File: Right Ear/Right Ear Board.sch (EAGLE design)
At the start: 6 parts, among them J1 502585-0470

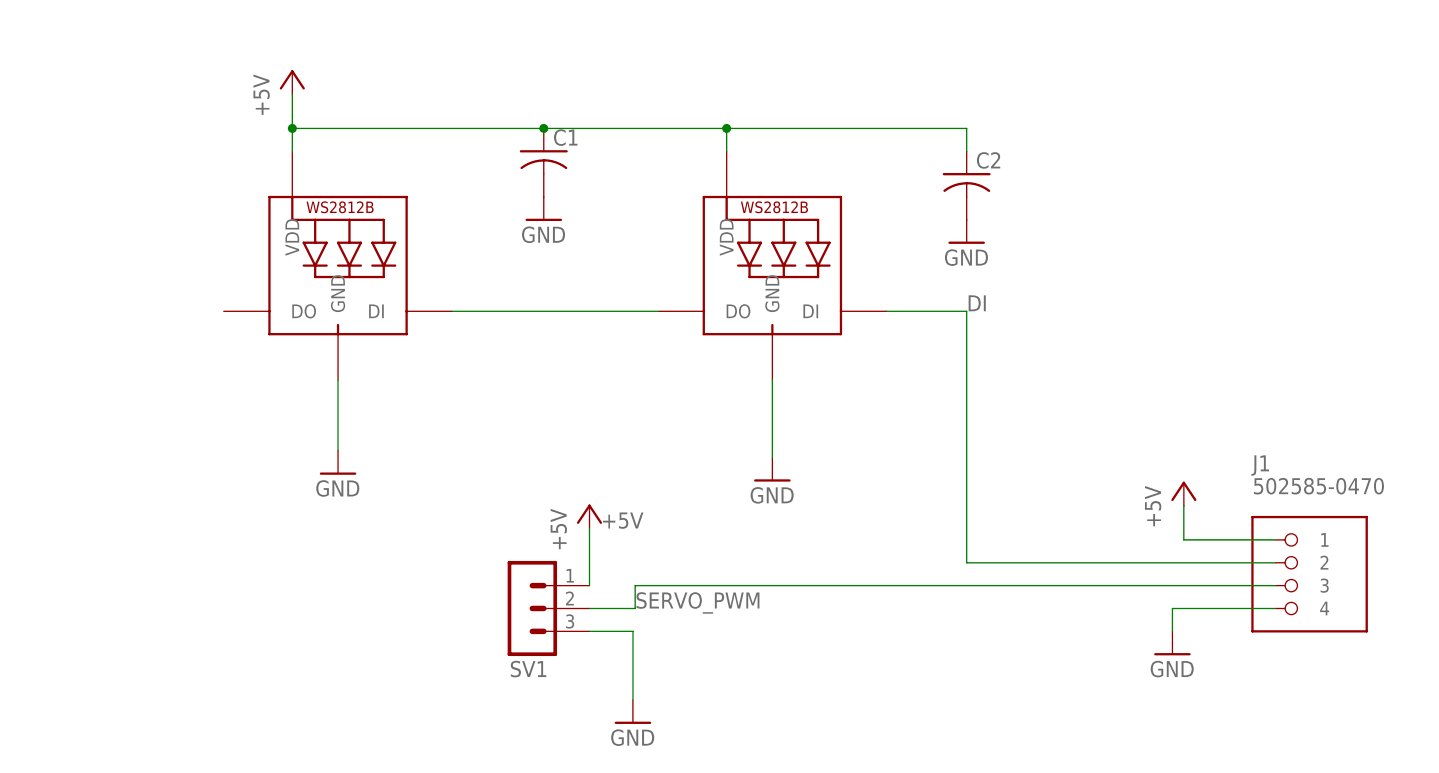
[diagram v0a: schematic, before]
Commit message: Update right ear boards
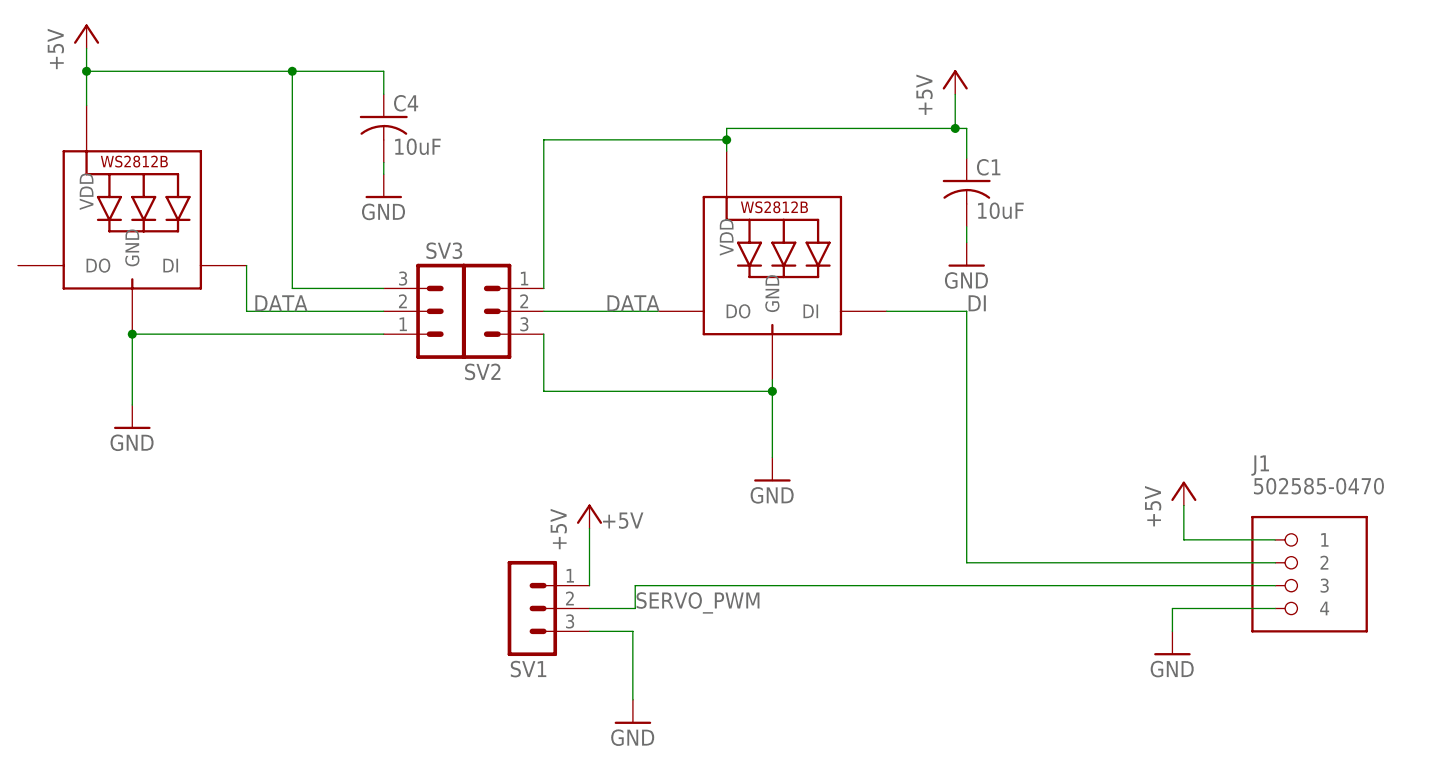
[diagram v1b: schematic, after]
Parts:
- removed C2: (no value), rcl:C-USC0402
- added C4: 10uF, rcl:C-USC0603K
- added SV2, SV3: (no value), con-lstb:MA03-1
- C1: value (none) -> 10uF; device rcl:C-USC0402 -> rcl:C-USC0603K; PARTNO (none) -> GRM188R61A106KE69D
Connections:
- removed net N$1: LED1.DO, LED7.DI
- new net DATA: LED1.DO, LED7.DI, SV2.2, SV3.2
- net +5V: now also C4.1, SV2.1, SV3.3; no longer C2.1
- net GND: now also C4.2, SV2.3, SV3.1; no longer C2.2
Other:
- moved on the sheet: C1
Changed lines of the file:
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@@
 <?xml version="1.0" encoding="utf-8"?>
 <!DOCTYPE eagle SYSTEM "eagle.dtd">
-<eagle version="8.6.0">
+<eagle version="8.5.0">
 <drawing>
 <settings>
@@
 <part name="LED7" library="adafruit" deviceset="WS2812B" device="5050"/>
 <part name="LED1" library="adafruit" deviceset="WS2812B" device="5050"/>
-<part name="C1" library="rcl" library_urn="urn:adsk.eagle:library:334" deviceset="C-US" device="C0402" package3d_urn="urn:adsk.eagle:package:23626/1"/>
 <part name="GND20" library="supply1" deviceset="GND" device=""/>
-<part name="C2" library="rcl" library_urn="urn:adsk.eagle:library:334" deviceset="C-US" device="C0402" package3d_urn="urn:adsk.eagle:package:23626/1"/>
 <part name="GND1" library="supply1" deviceset="GND" device=""/>
 <part name="J1" library="FormE" deviceset="MOLEX_CLICKMATE-4-R/A" device="" value="502585-0470"/>
@@
 <part name="P+2" library="supply1" library_urn="urn:adsk.eagle:library:371" deviceset="+5V" device=""/>
 <part name="P+3" library="supply1" library_urn="urn:adsk.eagle:library:371" deviceset="+5V" device=""/>
+<part name="SV2" library="con-lstb" library_urn="urn:adsk.eagle:library:162" deviceset="MA03-1" device="" package3d_urn="urn:adsk.eagle:package:8339/1"/>
+<part name="SV3" library="con-lstb" library_urn="urn:adsk.eagle:library:162" deviceset="MA03-1" device="" package3d_urn="urn:adsk.eagle:package:8339/1"/>
+<part name="C4" library="rcl" deviceset="C-US" device="C0603K" value="10uF">
+<attribute name="PARTNO" value="GRM188R61A106KE69D"/>
+</part>
+<part name="C1" library="rcl" deviceset="C-US" device="C0603K" value="10uF">
+<attribute name="PARTNO" value="GRM188R61A106KE69D"/>
+</part>
+<part name="P+4" library="supply1" library_urn="urn:adsk.eagle:library:371" deviceset="+5V" device=""/>
 </parts>
 <sheets>
@@
 <instances>
 <instance part="SV1" gate="G$1" x="78.74" y="46.99" rot="MR180"/>
-<instance part="LED7" gate="G$1" x="58.42" y="82.55" rot="MR0"/>
+<instance part="LED7" gate="G$1" x="35.56" y="87.63" rot="MR0"/>
 <instance part="LED1" gate="G$1" x="106.68" y="82.55" rot="MR0"/>
-<instance part="C1" gate="G$1" x="81.28" y="97.79"/>
-<instance part="GND20" gate="1" x="81.28" y="90.17"/>
-<instance part="C2" gate="G$1" x="128.27" y="95.25"/>
-<instance part="GND1" gate="1" x="128.27" y="87.63"/>
+<instance part="GND20" gate="1" x="63.5" y="92.71"/>
+<instance part="GND1" gate="1" x="128.27" y="85.09"/>
 <instance part="J1" gate="G$1" x="165.1" y="49.53"/>
-<instance part="GND2" gate="1" x="58.42" y="61.976"/>
+<instance part="GND2" gate="1" x="35.56" y="67.056"/>
 <instance part="GND3" gate="1" x="106.68" y="61.214"/>
 <instance part="GND4" gate="1" x="91.186" y="34.29"/>
 <instance part="GND5" gate="1" x="151.13" y="41.91"/>
 <instance part="P+1" gate="1" x="152.4" y="60.96"/>
-<instance part="P+2" gate="1" x="53.34" y="106.68"/>
+<instance part="P+2" gate="1" x="30.48" y="111.76"/>
 <instance part="P+3" gate="1" x="86.36" y="58.42"/>
+<instance part="SV2" gate="G$1" x="73.66" y="80.01" rot="MR180"/>
+<instance part="SV3" gate="G$1" x="71.12" y="80.01" rot="MR0"/>
+<instance part="C4" gate="G$1" x="63.5" y="101.6">
+<attribute name="PARTNO" x="63.5" y="101.6" size="1.778" layer="96" display="off"/>
+</instance>
+<instance part="C1" gate="G$1" x="128.27" y="94.488">
+<attribute name="PARTNO" x="128.27" y="94.488" size="1.778" layer="96" display="off"/>
+</instance>
+<instance part="P+4" gate="1" x="127" y="106.68"/>
 </instances>
 <busses>
@@
 </segment>
 <segment>
-<pinref part="C1" gate="G$1" pin="1"/>
-<pinref part="LED7" gate="G$1" pin="VDD"/>
-<wire x1="53.34" y1="97.79" x2="53.34" y2="100.33" width="0.1524" layer="91"/>
-<wire x1="53.34" y1="100.33" x2="53.34" y2="104.14" width="0.1524" layer="91"/>
-<wire x1="81.28" y1="100.33" x2="53.34" y2="100.33" width="0.1524" layer="91"/>
-<junction x="53.34" y="100.33"/>
-<pinref part="LED1" gate="G$1" pin="VDD"/>
-<wire x1="101.6" y1="97.79" x2="101.6" y2="100.33" width="0.1524" layer="91"/>
-<wire x1="81.28" y1="100.33" x2="101.6" y2="100.33" width="0.1524" layer="91"/>
-<junction x="81.28" y="100.33"/>
-<junction x="101.6" y="100.33"/>
-<pinref part="C2" gate="G$1" pin="1"/>
-<wire x1="101.6" y1="100.33" x2="128.27" y2="100.33" width="0.1524" layer="91"/>
-<wire x1="128.27" y1="100.33" x2="128.27" y2="97.79" width="0.1524" layer="91"/>
-<pinref part="P+2" gate="1" pin="+5V"/>
-</segment>
-<segment>
 <pinref part="J1" gate="G$1" pin="1"/>
 <wire x1="162.56" y1="54.61" x2="152.4" y2="54.61" width="0.1524" layer="91"/>
@@
 <pinref part="P+1" gate="1" pin="+5V"/>
 </segment>
+<segment>
+<wire x1="128.27" y1="100.33" x2="128.27" y2="97.028" width="0.1524" layer="91"/>
+<wire x1="101.6" y1="100.33" x2="127" y2="100.33" width="0.1524" layer="91"/>
+<pinref part="LED1" gate="G$1" pin="VDD"/>
+<wire x1="127" y1="100.33" x2="128.27" y2="100.33" width="0.1524" layer="91"/>
+<wire x1="101.6" y1="97.79" x2="101.6" y2="99.06" width="0.1524" layer="91"/>
+<pinref part="SV2" gate="G$1" pin="1"/>
+<wire x1="101.6" y1="99.06" x2="101.6" y2="100.33" width="0.1524" layer="91"/>
+<wire x1="81.28" y1="82.55" x2="81.28" y2="99.06" width="0.1524" layer="91"/>
+<wire x1="81.28" y1="99.06" x2="101.6" y2="99.06" width="0.1524" layer="91"/>
+<junction x="101.6" y="99.06"/>
+<pinref part="C1" gate="G$1" pin="1"/>
+<pinref part="P+4" gate="1" pin="+5V"/>
+<wire x1="127" y1="104.14" x2="127" y2="100.33" width="0.1524" layer="91"/>
+<junction x="127" y="100.33"/>
+</segment>
+<segment>
+<pinref part="LED7" gate="G$1" pin="VDD"/>
+<pinref part="P+2" gate="1" pin="+5V"/>
+<wire x1="30.48" y1="102.87" x2="30.48" y2="106.68" width="0.1524" layer="91"/>
+<pinref part="C4" gate="G$1" pin="1"/>
+<wire x1="30.48" y1="106.68" x2="30.48" y2="109.22" width="0.1524" layer="91"/>
+<wire x1="63.5" y1="104.14" x2="63.5" y2="106.68" width="0.1524" layer="91"/>
+<wire x1="63.5" y1="106.68" x2="53.34" y2="106.68" width="0.1524" layer="91"/>
+<junction x="30.48" y="106.68"/>
+<pinref part="SV3" gate="G$1" pin="3"/>
+<wire x1="53.34" y1="106.68" x2="30.48" y2="106.68" width="0.1524" layer="91"/>
+<wire x1="63.5" y1="82.55" x2="53.34" y2="82.55" width="0.1524" layer="91"/>
+<wire x1="53.34" y1="82.55" x2="53.34" y2="106.68" width="0.1524" layer="91"/>
+<junction x="53.34" y="106.68"/>
+</segment>
 </net>
 <net name="GND" class="0">
-<segment>
-<pinref part="C1" gate="G$1" pin="2"/>
-<pinref part="GND20" gate="1" pin="GND"/>
-</segment>
-<segment>
-<pinref part="C2" gate="G$1" pin="2"/>
-<pinref part="GND1" gate="1" pin="GND"/>
-</segment>
 <segment>
 <pinref part="J1" gate="G$1" pin="4"/>
@@
 <pinref part="LED7" gate="G$1" pin="GND"/>
 <pinref part="GND2" gate="1" pin="GND"/>
-<wire x1="58.42" y1="72.39" x2="58.42" y2="64.516" width="0.1524" layer="91"/>
+<wire x1="35.56" y1="77.47" x2="35.56" y2="69.596" width="0.1524" layer="91"/>
+<pinref part="SV3" gate="G$1" pin="1"/>
+<wire x1="63.5" y1="77.47" x2="35.56" y2="77.47" width="0.1524" layer="91"/>
+<junction x="35.56" y="77.47"/>
 </segment>
 <segment>
 <pinref part="LED1" gate="G$1" pin="GND"/>
 <pinref part="GND3" gate="1" pin="GND"/>
-<wire x1="106.68" y1="72.39" x2="106.68" y2="63.754" width="0.1524" layer="91"/>
+<wire x1="106.68" y1="72.39" x2="106.68" y2="71.12" width="0.1524" layer="91"/>
+<pinref part="SV2" gate="G$1" pin="3"/>
+<wire x1="106.68" y1="71.12" x2="106.68" y2="63.754" width="0.1524" layer="91"/>
+<wire x1="81.28" y1="77.47" x2="81.28" y2="71.12" width="0.1524" layer="91"/>
+<wire x1="81.28" y1="71.12" x2="106.68" y2="71.12" width="0.1524" layer="91"/>
+<junction x="106.68" y="71.12"/>
 </segment>
 <segment>
@@
 <wire x1="86.36" y1="44.45" x2="91.186" y2="44.45" width="0.1524" layer="91"/>
 <wire x1="91.186" y1="44.45" x2="91.186" y2="36.83" width="0.1524" layer="91"/>
+</segment>
+<segment>
+<pinref part="GND20" gate="1" pin="GND"/>
+<pinref part="C4" gate="G$1" pin="2"/>
+<wire x1="63.5" y1="95.25" x2="63.5" y2="96.52" width="0.1524" layer="91"/>
+</segment>
+<segment>
+<pinref part="C1" gate="G$1" pin="2"/>
+<pinref part="GND1" gate="1" pin="GND"/>
+<wire x1="128.27" y1="89.408" x2="128.27" y2="87.63" width="0.1524" layer="91"/>
 </segment>
 </net>
@@
 </segment>
 </net>
-<net name="N$1" class="0">
-<segment>
+<net name="DATA" class="0">
+<segment>
+<pinref part="LED1" gate="G$1" pin="DO"/>
+<pinref part="SV2" gate="G$1" pin="2"/>
+<wire x1="93.98" y1="80.01" x2="81.28" y2="80.01" width="0.1524" layer="91"/>
+<label x="88.138" y="80.01" size="1.778" layer="95"/>
+</segment>
+<segment>
+<pinref part="SV3" gate="G$1" pin="2"/>
 <pinref part="LED7" gate="G$1" pin="DI"/>
-<pinref part="LED1" gate="G$1" pin="DO"/>
-<wire x1="71.12" y1="80.01" x2="93.98" y2="80.01" width="0.1524" layer="91"/>
-</segment>
-</net>
+<wire x1="63.5" y1="80.01" x2="48.26" y2="80.01" width="0.1524" layer="91"/>
+<wire x1="48.26" y1="80.01" x2="48.26" y2="85.09" width="0.1524" layer="91"/>
+<label x="49.022" y="80.01" size="1.778" layer="95"/>
+</segment>
+</net>
